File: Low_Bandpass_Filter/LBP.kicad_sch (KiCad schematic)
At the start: 40 parts, among them IC1 OPA1644AIPWR, U1 OPA1641, U2 OPA1641, U3 OPA1641, U4 OPA1641

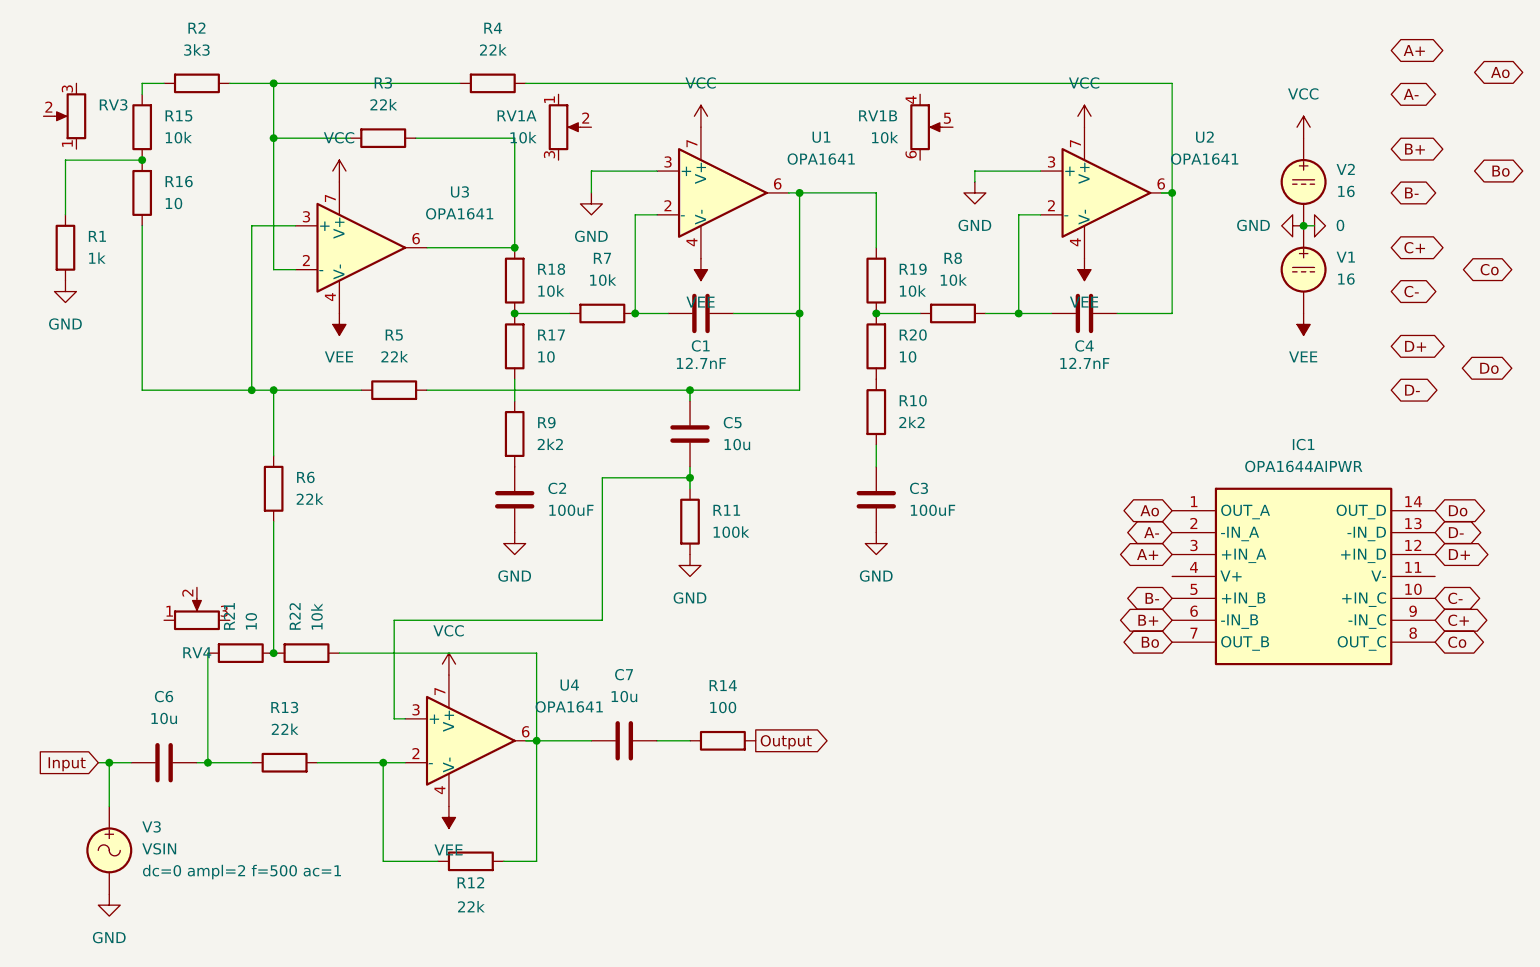
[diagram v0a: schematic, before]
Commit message: started main schematic
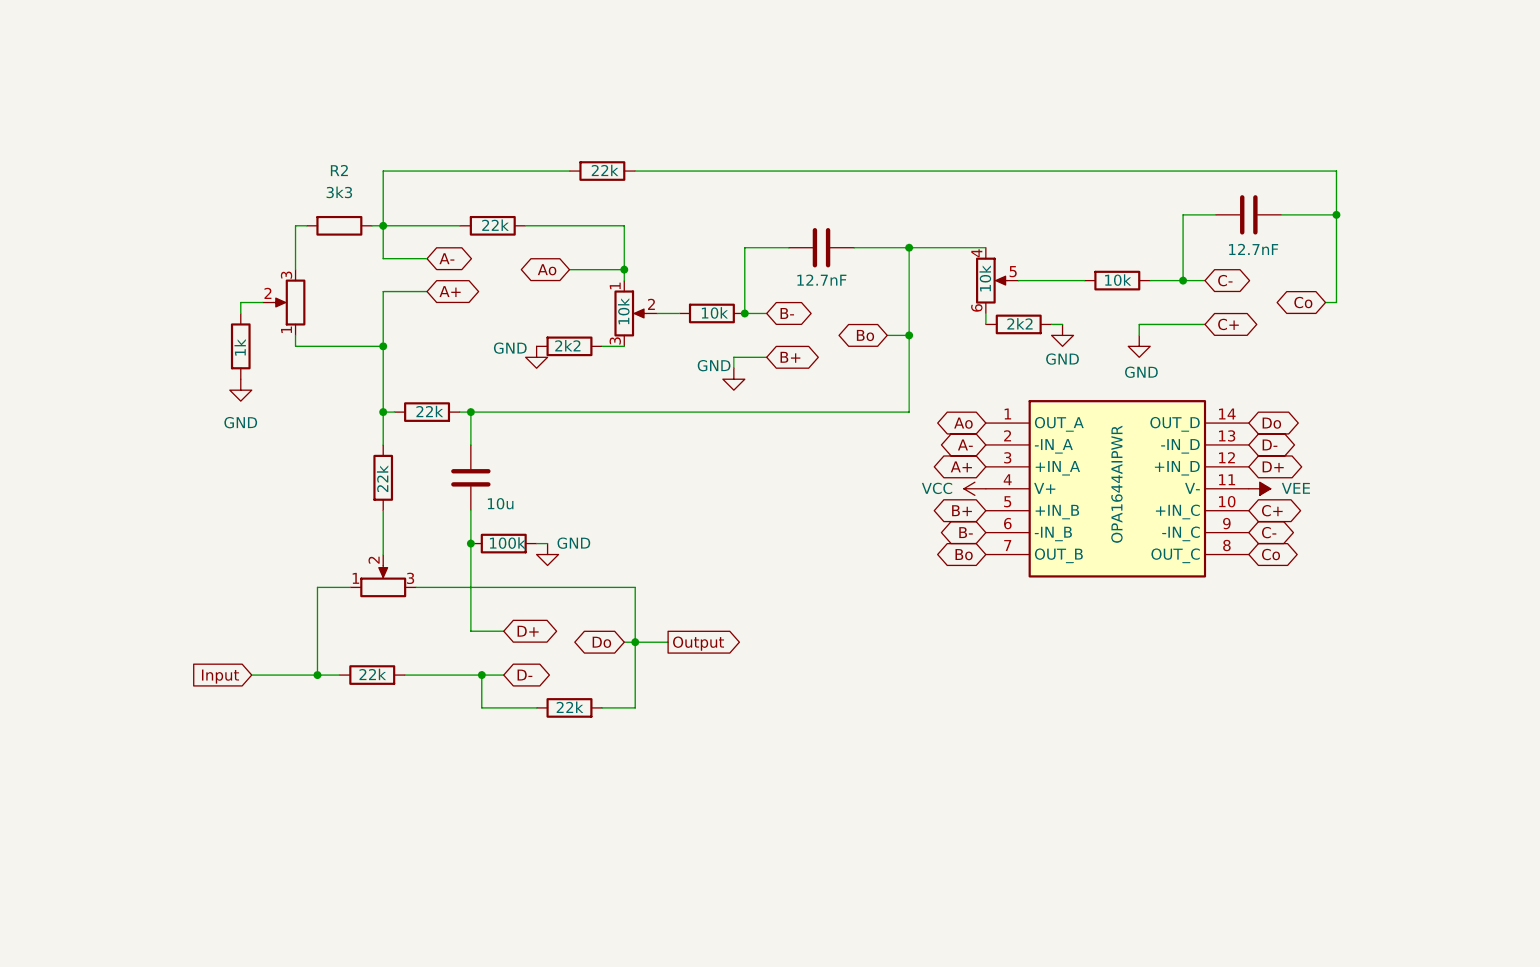
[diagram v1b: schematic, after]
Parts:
- removed C2, C3: 100uF, symbol Device:C
- removed C6, C7: 10u, symbol Device:C
- removed R14: 100, Resistor_THT:R_Axial_DIN0207_L6.3mm_D2.5mm_P10.16mm_Horizontal, symbol Device:R
- removed R15, R18, R19, R22: 10k, Resistor_THT:R_Axial_DIN0207_L6.3mm_D2.5mm_P10.16mm_Horizontal, symbol Device:R
- removed R16, R17, R20, R21: 10, Resistor_THT:R_Axial_DIN0207_L6.3mm_D2.5mm_P10.16mm_Horizontal, symbol Device:R
- removed U1, U2, U3, U4: OPA1641, OPA1641:OPA1641, symbol Amplifier_Operational:OPA1641
- removed V1, V2: 16, symbol Simulation_SPICE:VDC
- removed V3: VSIN, symbol Simulation_SPICE:VSIN
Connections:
- net 0 is gone; now on net GND: R1.2, R11.2
- net B+ is gone; now on net B-: IC1.6 (-IN_B)
- net C+ is gone; now on net C-: IC1.9 (-IN_C)
- net A+: now also R5.1, R6.1, RV3.1
- net A-: now also R2.1, R3.2, R4.2
- net Ao: now also R3.1, RV1.1
- net B-: now also C1.1, R7.1; no longer IC1.5 (+IN_B)
- net Bo: now also C1.2, C5.2, R5.2, RV1.4
- net C-: now also C4.1, R8.1; no longer IC1.10 (+IN_C)
- net Co: now also C4.2, R4.1
- net D+: now also C5.1, R11.1
- net D-: now also R12.1, R13.2
- net Do: now also R12.2, RV4.3
- net Input: now also R13.1, RV4.1
- net VCC: now also IC1.4 (V+)
- net VEE: now also IC1.11 (V-)
- net at RV1.5: now also R8.2
- net at RV1.6: now also R10.1
- net at RV1.2: now also R7.2
- net at RV1.3: now also R9.1
- net at R6.2: now also RV4.2
- net at R1.1: now also RV3.2
- net at R2.2: now also RV3.3
- net GND: now reaches R9.2
- net GND: now also IC1.10 (+IN_C), IC1.5 (+IN_B), R10.2
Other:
- moved on the sheet: R2
